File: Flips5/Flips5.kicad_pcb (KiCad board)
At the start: 2 copper layers, 100 x 100 mm, 24 parts, among them IC1 FP2800A, IC2 FP2800A, IC3 FP2800A

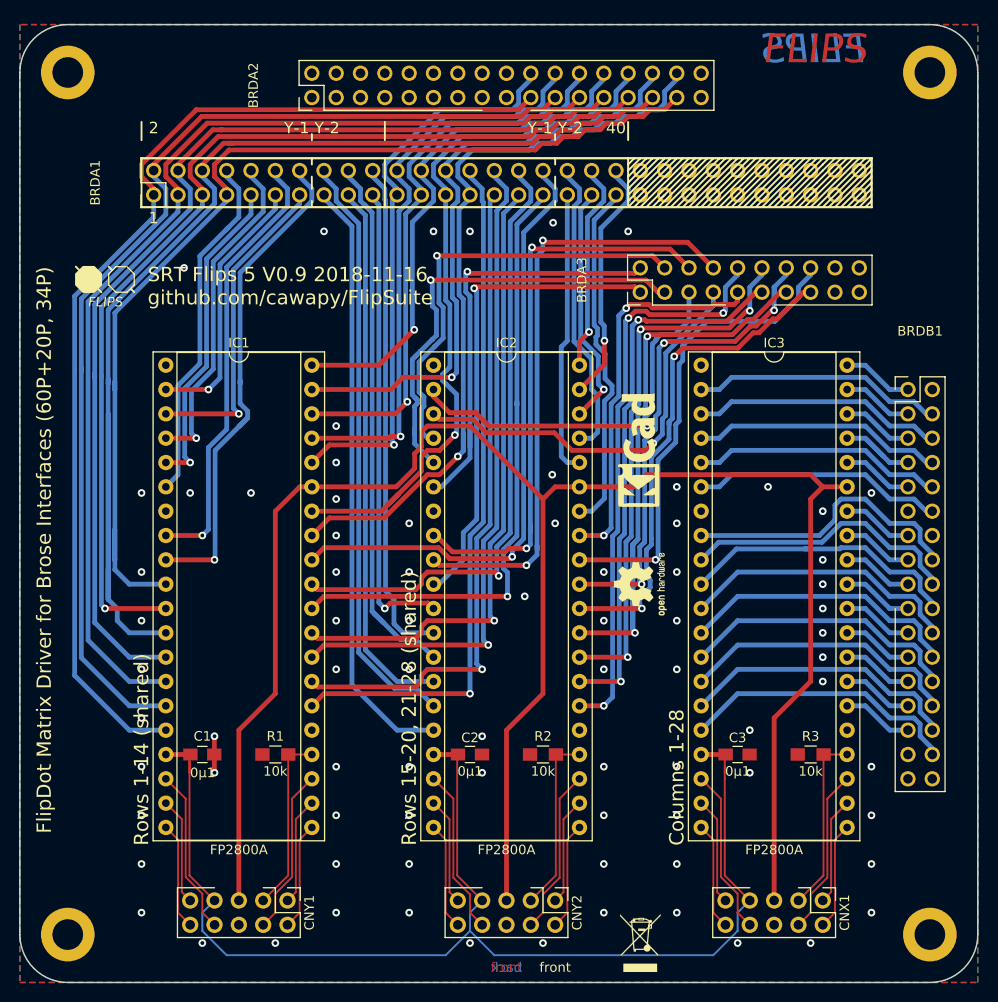
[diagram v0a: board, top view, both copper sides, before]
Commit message: sorting traces
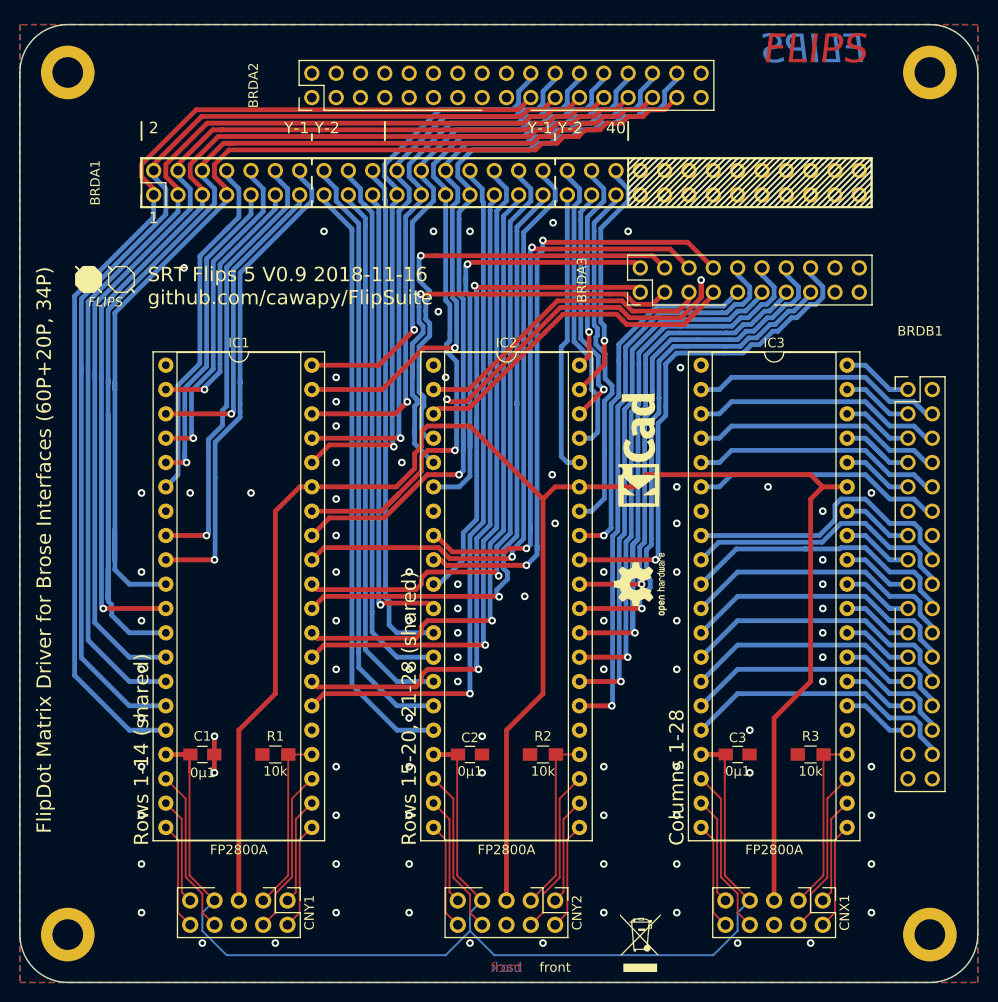
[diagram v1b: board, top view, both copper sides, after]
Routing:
- net /GND: track 3.91 -> 39.5 mm, vias 80 -> 93
- net /SY25: track 41.2 -> 32.3 mm, vias 1 -> 0
- net /~RY21: track 42.1 -> 37.8 mm, vias 2 -> 1
- net /SY27: track 43.2 -> 39.6 mm, vias 1 -> 0
- net /~RY28: track 49.3 -> 51.7 mm
- net /SY22: track 45.1 -> 47.2 mm
- net /~RY27: track 52.0 -> 53.9 mm, vias 2 -> 1
- net /SY23: track 47.8 -> 49.6 mm
- net /SY14: track 52.6 -> 50.8 mm
- net /SY24: track 45.9 -> 47.6 mm
- net /~RY6: track 65.3 -> 63.7 mm
- net /SY21: track 52.2 -> 53.7 mm
- net /~RY23: track 57.2 -> 55.8 mm, vias 2 -> 1
- net /~RY7: track 79.5 -> 81.0 mm
- net /SY19: track 49.3 -> 50.6 mm
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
